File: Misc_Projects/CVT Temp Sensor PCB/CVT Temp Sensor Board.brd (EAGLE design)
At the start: 160 x 100 mm, 2 parts, among them IC1 TSD305-1SL10

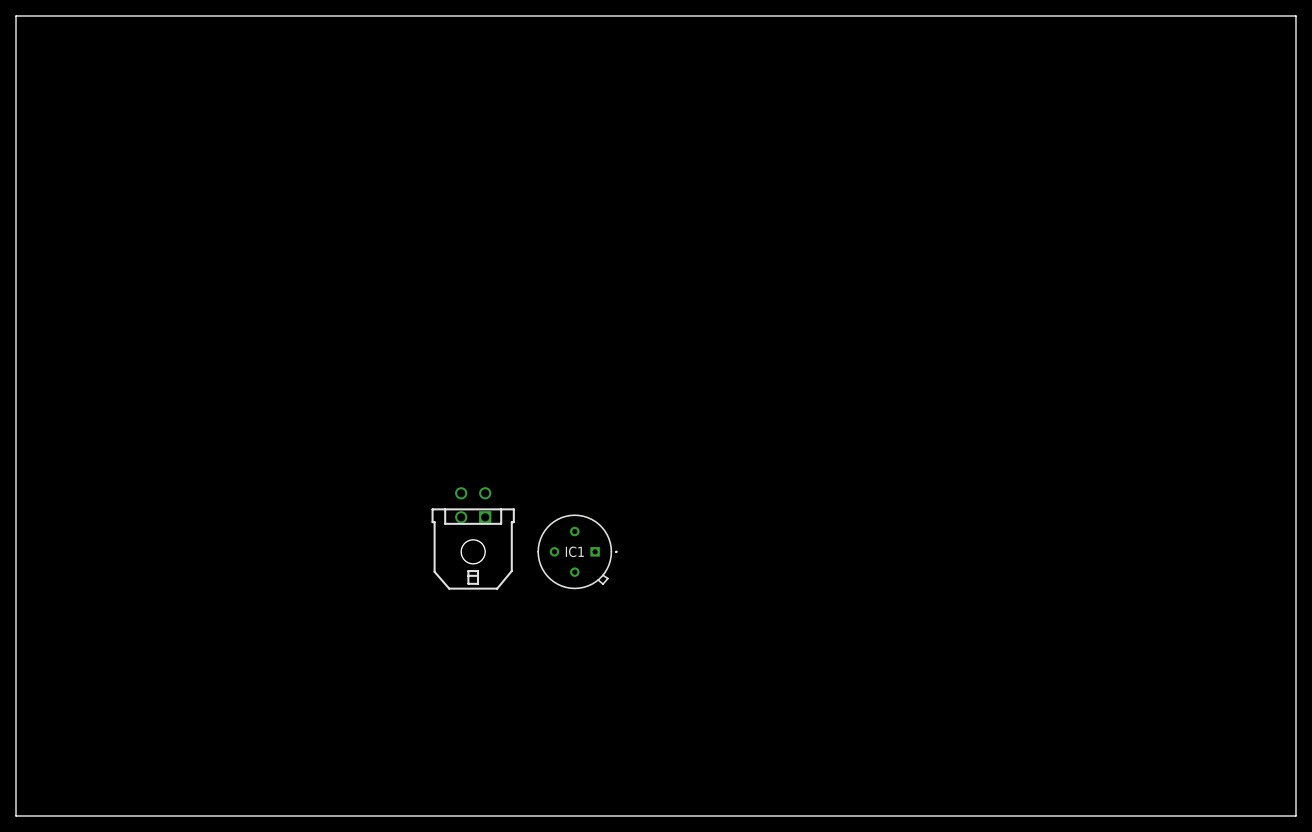
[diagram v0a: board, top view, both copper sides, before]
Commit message: CVT Temp Board Sensor PCB
Version 1.1
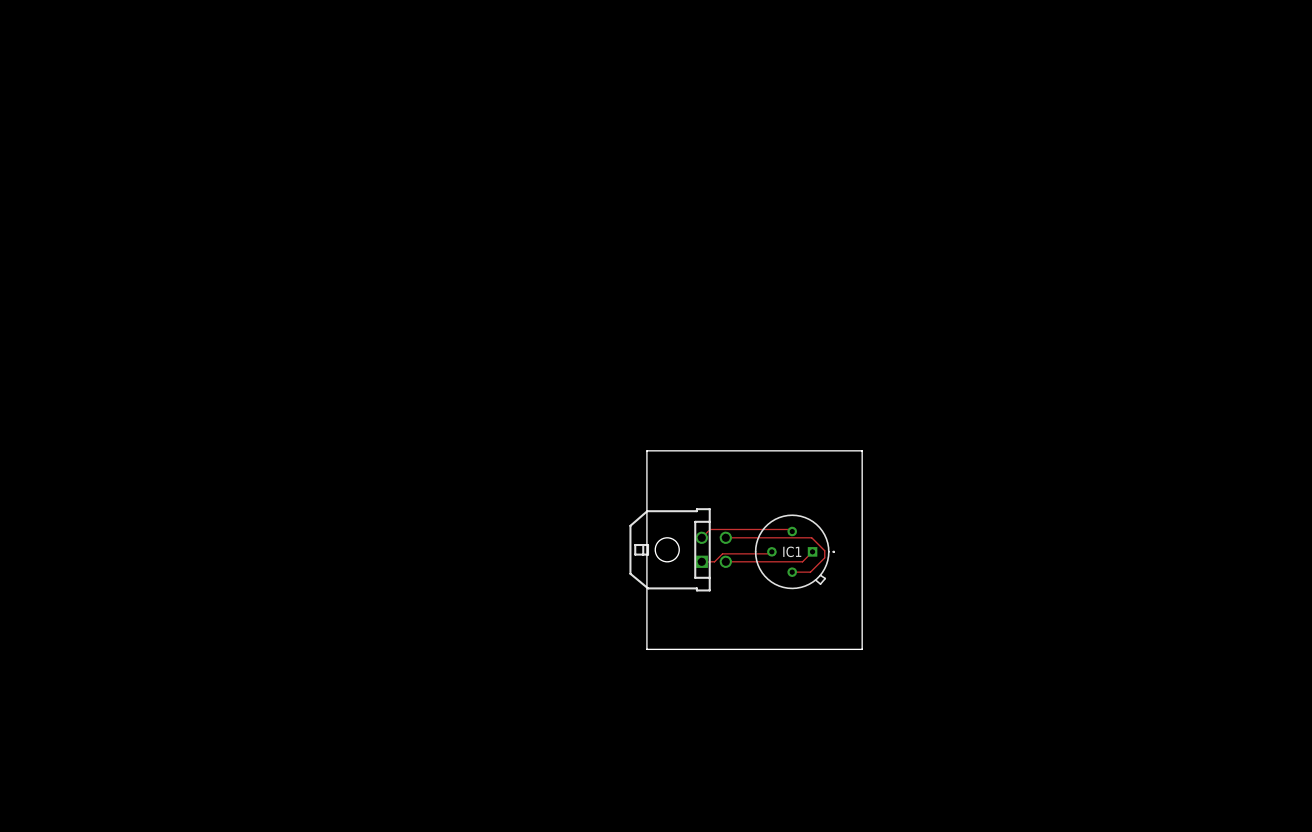
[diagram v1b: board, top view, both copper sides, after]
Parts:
- moved IC1 27.2 mm to (99.6, 33.0)
- moved X1 24.3 mm to (81.4, 33.3), turned to 270 degrees
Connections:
- removed net N$2: X1.P$2
- removed net N$3: X1.P$3
- new net SCL: IC1.1, X1.P$3
- new net SDA: IC1.2, X1.P$2
- net +3V3: now also IC1.3
- net GND: now also IC1.4
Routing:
- net GND: track 0.00 -> 18.7 mm
- net SDA: track 0.00 -> 11.8 mm
- net SCL: track 0.00 -> 11.4 mm
- net +3V3: track 0.00 -> 9.28 mm
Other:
- board size 160 x 100 mm -> 26.9 x 24.8 mm
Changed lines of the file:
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@@
 <setting verticaltext="up"/>
 </settings>
-<grid distance="50" unitdist="mil" unit="mil" style="lines" multiple="1" display="no" altdistance="5" altunitdist="mil" altunit="mil"/>
+<grid distance="5" unitdist="mil" unit="mil" style="lines" multiple="1" display="yes" altdistance="5" altunitdist="mil" altunit="mil"/>
 <layers>
 <layer number="1" name="Top" color="4" fill="1" visible="yes" active="yes"/>
@@
 <board>
 <plain>
-<wire x1="0" y1="0" x2="160" y2="0" width="0" layer="20"/>
-<wire x1="160" y1="0" x2="160" y2="100" width="0" layer="20"/>
-<wire x1="160" y1="100" x2="0" y2="100" width="0" layer="20"/>
-<wire x1="0" y1="100" x2="0" y2="0" width="0" layer="20"/>
+<wire x1="78.867" y1="20.828" x2="105.771" y2="20.828" width="0" layer="20"/>
+<wire x1="105.771" y1="20.828" x2="105.771" y2="45.644" width="0" layer="20"/>
+<wire x1="105.771" y1="45.644" x2="78.867" y2="45.644" width="0" layer="20"/>
+<wire x1="78.867" y1="45.644" x2="78.867" y2="20.828" width="0" layer="20"/>
 </plain>
 <attributes>
@@
 </autorouter>
 <elements>
-<element name="IC1" library="TSD305-1SL10" package="TSD3051SL10" value="TSD305-1SL10" x="72.39" y="33.02" smashed="yes">
-<attribute name="DESCRIPTION" value="Board Mount Temperature Sensors TO5, I2C Interrface 0 C to +300 C" x="90.17" y="26.67" size="1.778" layer="27" display="off"/>
-<attribute name="HEIGHT" value="8.65mm" x="90.17" y="26.67" size="1.778" layer="27" display="off"/>
-<attribute name="MANUFACTURER_NAME" value="TE Connectivity" x="90.17" y="26.67" size="1.778" layer="27" display="off"/>
-<attribute name="MANUFACTURER_PART_NUMBER" value="TSD305-1SL10" x="90.17" y="26.67" size="1.778" layer="27" display="off"/>
-<attribute name="MOUSER_PART_NUMBER" value="824-TSD305-1SL10" x="90.17" y="26.67" size="1.778" layer="27" display="off"/>
-<attribute name="MOUSER_PRICE-STOCK" value="https://www.mouser.co.uk/ProductDetail/Measurement-Specialties/TSD305-1SL10?qs=l7cgNqFNU1hQbECGfV0ZYg%3D%3D" x="90.17" y="26.67" size="1.778" layer="27" display="off"/>
-<attribute name="NAME" x="69.85" y="33.02" size="1.27" layer="25" align="center"/>
-<attribute name="VALUE" x="69.85" y="40.64" size="1.27" layer="27" align="center"/>
+<element name="IC1" library="TSD305-1SL10" package="TSD3051SL10" value="TSD305-1SL10" x="99.568" y="33.02" smashed="yes">
+<attribute name="DESCRIPTION" value="Board Mount Temperature Sensors TO5, I2C Interrface 0 C to +300 C" x="117.348" y="26.67" size="1.778" layer="27" display="off"/>
+<attribute name="HEIGHT" value="8.65mm" x="117.348" y="26.67" size="1.778" layer="27" display="off"/>
+<attribute name="MANUFACTURER_NAME" value="TE Connectivity" x="117.348" y="26.67" size="1.778" layer="27" display="off"/>
+<attribute name="MANUFACTURER_PART_NUMBER" value="TSD305-1SL10" x="117.348" y="26.67" size="1.778" layer="27" display="off"/>
+<attribute name="MOUSER_PART_NUMBER" value="824-TSD305-1SL10" x="117.348" y="26.67" size="1.778" layer="27" display="off"/>
+<attribute name="MOUSER_PRICE-STOCK" value="https://www.mouser.co.uk/ProductDetail/Measurement-Specialties/TSD305-1SL10?qs=l7cgNqFNU1hQbECGfV0ZYg%3D%3D" x="117.348" y="26.67" size="1.778" layer="27" display="off"/>
+<attribute name="NAME" x="97.028" y="33.02" size="1.27" layer="25" rot="R180" align="center"/>
+<attribute name="VALUE" x="97.409" y="40.005" size="1.27" layer="27" align="center"/>
 </element>
-<element name="X1" library="GTOR - Microfit Connector" package="43045-0400" value="" x="57.15" y="33.02" smashed="yes">
-<attribute name="MATERIAL" value="" x="57.15" y="33.02" size="1.778" layer="27" display="off"/>
+<element name="X1" library="GTOR - Microfit Connector" package="43045-0400" value="" x="81.407" y="33.274" smashed="yes" rot="R270">
+<attribute name="MATERIAL" value="" x="81.407" y="33.274" size="1.778" layer="27" rot="R270" display="off"/>
 </element>
 </elements>
@@
 <signal name="+3V3">
 <contactref element="X1" pad="P$1"/>
+<contactref element="IC1" pad="3"/>
+<wire x1="85.727" y1="31.774" x2="87.32183125" y2="31.774" width="0.1524" layer="1"/>
+<wire x1="87.32183125" y1="31.774" x2="88.31543125" y2="32.7676" width="0.1524" layer="1"/>
+<wire x1="94.2356" y1="32.7676" x2="94.488" y2="33.02" width="0.1524" layer="1"/>
+<wire x1="88.31543125" y1="32.7676" x2="94.2356" y2="32.7676" width="0.1524" layer="1"/>
 </signal>
-<signal name="N$2">
+<signal name="SDA">
 <contactref element="X1" pad="P$2"/>
+<contactref element="IC1" pad="2"/>
+<wire x1="85.727" y1="34.774" x2="86.767" y2="35.814" width="0.1524" layer="1"/>
+<wire x1="96.774" y1="35.814" x2="86.767" y2="35.814" width="0.1524" layer="1"/>
+<wire x1="96.774" y1="35.814" x2="97.028" y2="35.56" width="0.1524" layer="1"/>
 </signal>
-<signal name="N$3">
+<signal name="SCL">
 <contactref element="X1" pad="P$3"/>
+<contactref element="IC1" pad="1"/>
+<wire x1="88.727" y1="31.774" x2="98.322" y2="31.774" width="0.1524" layer="1"/>
+<wire x1="98.322" y1="31.774" x2="99.568" y2="33.02" width="0.1524" layer="1"/>
 </signal>
 <signal name="GND">
 <contactref element="X1" pad="P$4"/>
+<contactref element="IC1" pad="4"/>
+<wire x1="88.727" y1="34.774" x2="99.465" y2="34.774" width="0.1524" layer="1"/>
+<wire x1="99.465" y1="34.774" x2="101.092" y2="33.147" width="0.1524" layer="1"/>
+<wire x1="101.092" y1="33.147" x2="101.092" y2="32.258" width="0.1524" layer="1"/>
+<wire x1="101.092" y1="32.258" x2="99.314" y2="30.48" width="0.1524" layer="1"/>
+<wire x1="99.314" y1="30.48" x2="97.028" y2="30.48" width="0.1524" layer="1"/>
 </signal>
 </signals>
